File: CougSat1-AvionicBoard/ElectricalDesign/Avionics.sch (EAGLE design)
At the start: 165 parts, among them J11 -Y, J12 +Z, J13 +X, J14 -Z, J15 +Y, J3 SWD, J4 CougSat Card, J5 -X, J8 SWD, J9 SWD, U1 STM32L476RGT, U10 BNO055, U11 128KB, U12 TXS0102DQM, U13 TXS0102DQM, U14 LTC2499, U15 BNO055, U16 BNO055, U17 TXS0102DQM, U18 TXS0102DQM, U2 STM32L476RGT, U3 STM32L476RGT, U4 128KB, U5 DRV8837, U6 DRV8837, U7 DRV8837, U8 LTC2499, U9 Venus838FLPx-L, Y1 16MHz ±10ppm, Y10 16MHz ±10ppm, Y2 32.768kHz ±10ppm, Y3 16MHz ±10ppm, Y4 32.768kHz ±10ppm, Y6 32.768kHz ±10ppm, Y7 32.768kHz ±10ppm, Y8 32.768kHz ±10ppm, Y9 32.768kHz ±10ppm

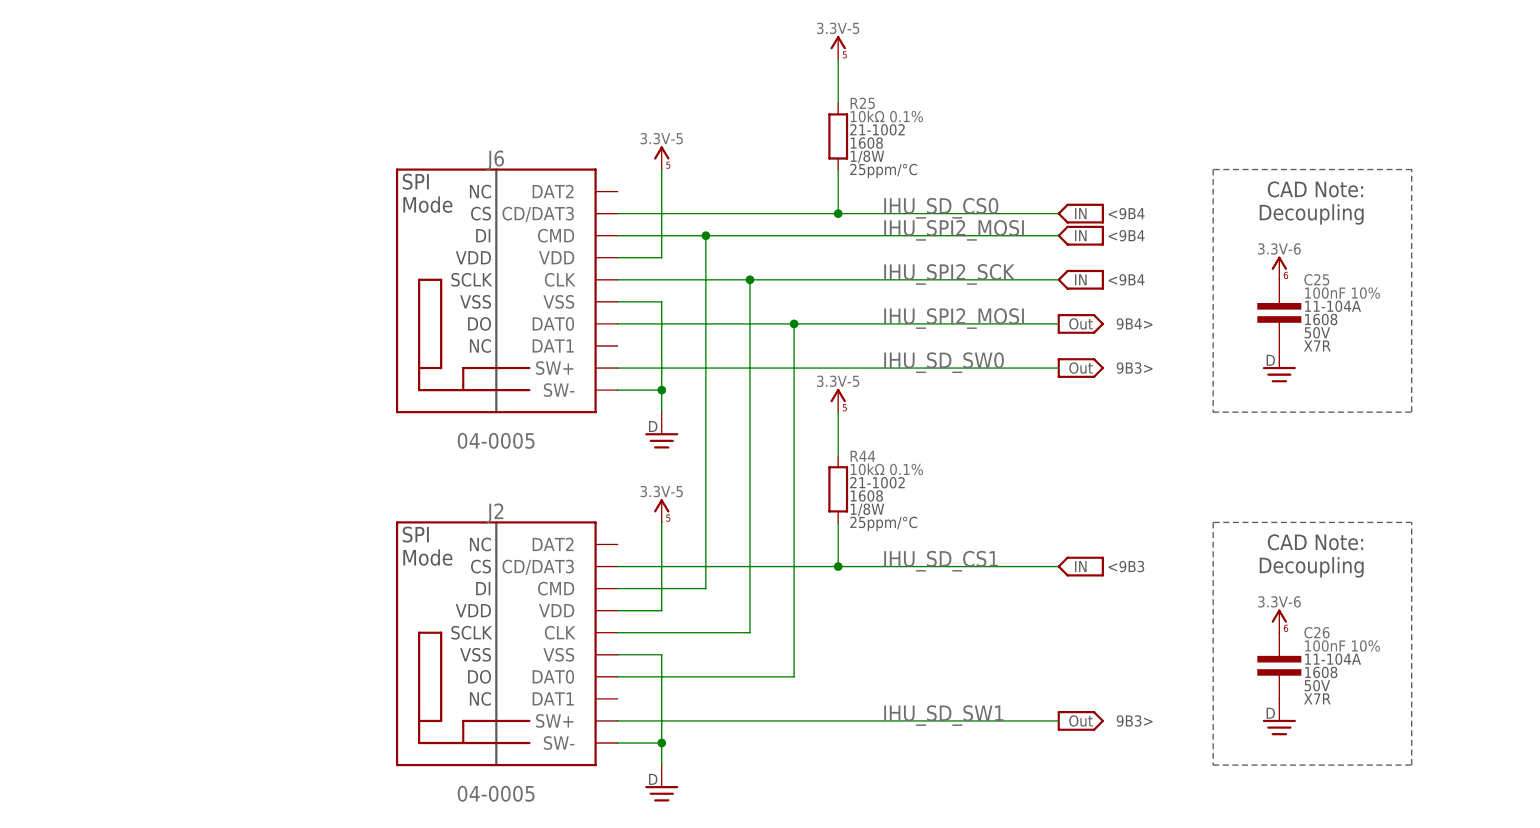
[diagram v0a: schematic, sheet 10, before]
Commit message: Updated Thermistors
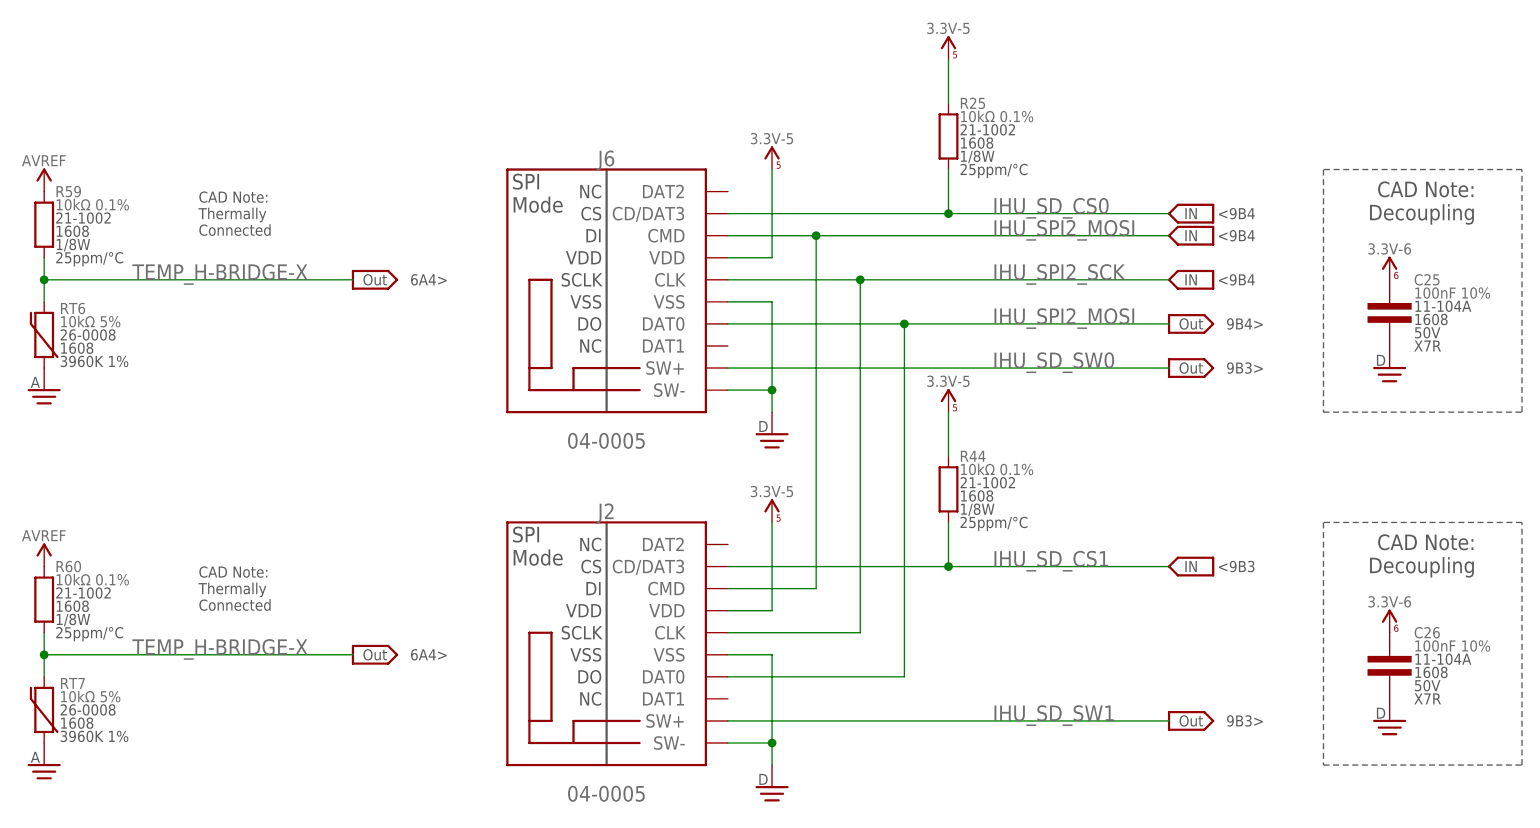
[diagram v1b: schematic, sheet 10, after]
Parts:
- removed RT12, RT13, RT14: 68kΩ 5%, CougsInSpace-Resistors:THERMISTOR-H-68K-1608
- added R47, R48, R49, R50, R51, R52, R53, R54, R55, R56, R57, R58, R59, R60: 10kΩ 0.1%, CougsInSpace-Resistors:RES-V-10K-1608
- added RT15, RT16, RT17, RT18: 10kΩ 5%, CougsInSpace-Resistors:THERMISTOR-V-10K-1608
- RT1, RT10, RT2, RT3, RT4, RT5, RT6, RT7, RT8, RT9: value 68kΩ 5% -> 10kΩ 5%; device CougsInSpace-Resistors:THERMISTOR-H-68K-1608 -> CougsInSpace-Resistors:THERMISTOR-V-10K-1608
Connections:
- net AGND: now also RT1.1, RT10.1, RT15.1, RT16.1, RT17.1, RT18.1, RT2.1, RT3.1, RT4.1, RT5.1, RT6.1, RT7.1, RT8.1, RT9.1
- net AVDD: no longer RT1.2, RT10.2, RT12.2, RT13.2, RT14.2, RT2.2, RT3.2, RT4.2, RT5.2, RT6.2, RT7.2, RT8.2, RT9.2
- net AVREF: now also R47.2, R48.2, R49.2, R50.2, R51.2, R52.2, R53.2, R54.2, R55.2, R56.2, R57.2, R58.2, R59.2, R60.2
- net TEMP_ADCS: now also R47.1, RT15.2
- net TEMP_GPS: now also R54.1, RT1.2; no longer RT1.1
- net TEMP_H-BRIDGE-X: now also R51.1, R59.1, R60.1, RT6.2, RT7.2, RT8.2; no longer RT3.1
- net TEMP_H-BRIDGE-Y: now also R52.1, RT9.2; no longer RT4.1
- net TEMP_H-BRIDGE-Z: now also R53.1, RT10.2; no longer RT5.1
- net TEMP_IFJR: now also R55.1, RT3.2; no longer RT2.1
- net TEMP_IHU: now also R58.1, RT5.2; no longer RT14.1
- net TEMP_IMU0: now also R48.1, RT16.2; no longer RT8.1
- net TEMP_IMU1: now also R49.1, RT17.2; no longer RT9.1
- net TEMP_IMU2: now also R50.1, RT18.2; no longer RT10.1
- net TEMP_SD_IFJR0: now also R56.1, RT2.2; no longer RT6.1
- net TEMP_SD_IFJR1: now also R57.1, RT4.2; no longer RT7.1
- net TEMP_SD_IHU0: no longer RT12.1
- net TEMP_SD_IHU1: no longer RT13.1
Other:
- note added: "4A5>"
- note added: "6A2>"
- note added: "6A4>"
- note added: "<3A6"
- note added: "<4A5"
- note added: "<4A6"
- note added: "<5A6"
- note added: "<5B6"
- note added: "<5C6"
- note removed: "<3A5"
- note removed: "<4A1"
- note removed: "<5B2"
- note removed: "<5C2"
- note removed: "<5D2"
- note removed: "<6A2"
- note removed: "<6A4"
- note removed: "<6B2"
- note removed: "<6C2"
- moved on the sheet: C25, C26, DS3, DS5, J2, J6, J9, R25, R27, R38, R44, R46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
